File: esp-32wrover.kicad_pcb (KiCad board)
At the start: 2 copper layers, 68.6 x 53.3 mm, 8 parts, among them P1 Power, P2 Analog, P3 Digital, P4 Digital, P5 CONN_1, P6 CONN_1, P7 CONN_1, P8 CONN_1

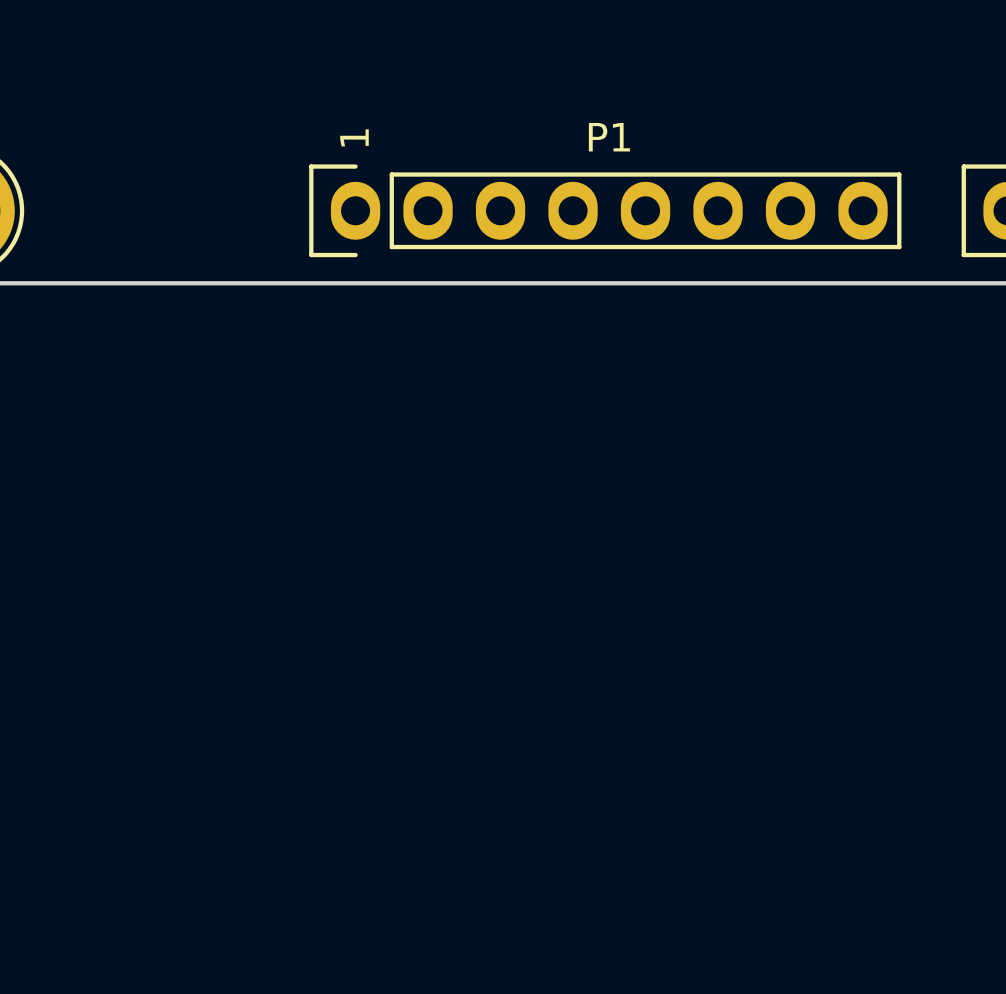
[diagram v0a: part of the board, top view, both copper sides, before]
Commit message: edit netlist, create pcb
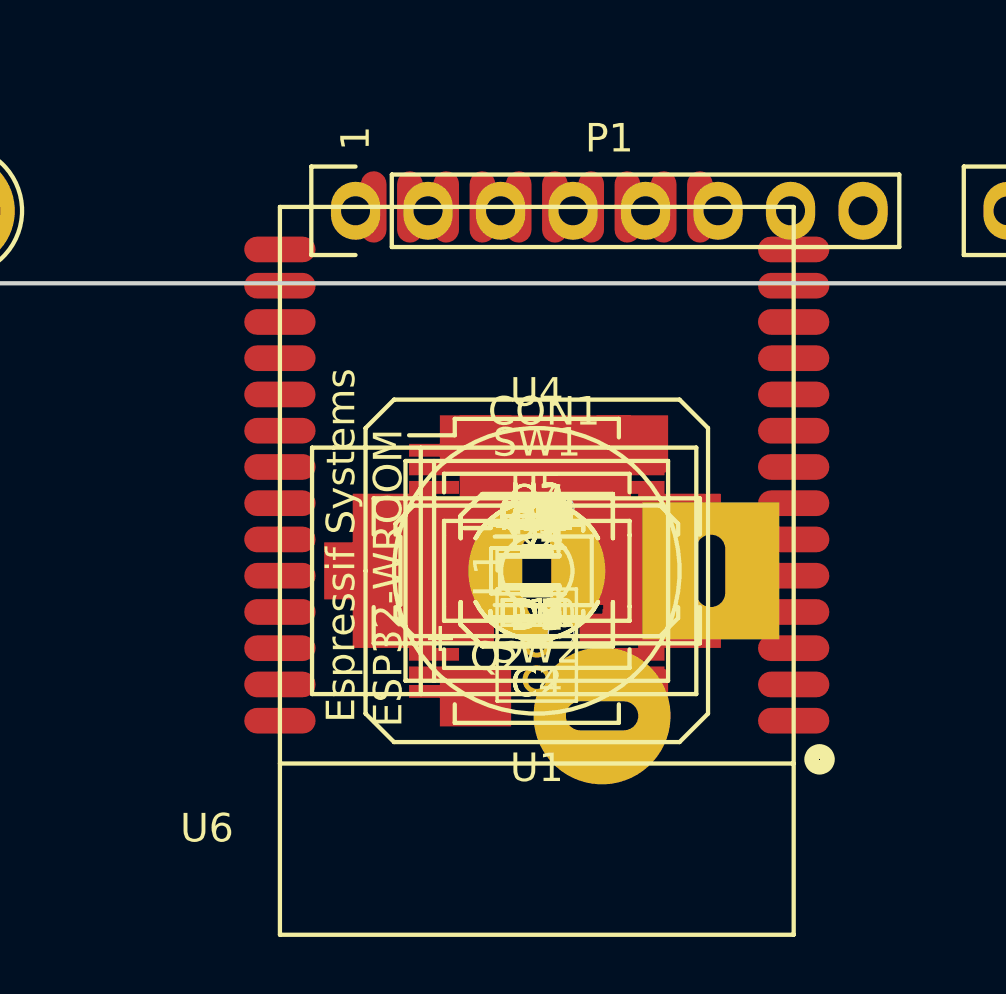
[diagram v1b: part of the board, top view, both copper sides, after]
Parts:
- added C1, C3: 1nF/50V, Capacitors_SMD:C_0603, F.Cu at (145.3, 136.4)
- added C10: 1uF, Capacitors_SMD:C_0805, F.Cu at (145.3, 136.4)
- added C11, C13, C14, C16, C17: C, Capacitors_SMD:C_0603, F.Cu at (145.3, 136.4)
- added C12, C15: 10uF/25V, Capacitors_SMD:C_0603, F.Cu at (145.3, 136.4)
- added C18: 1uF/25V, Capacitors_SMD:C_0603, F.Cu at (145.3, 136.4)
- added C19, C20: 0.1uF, Capacitors_SMD:C_0603, F.Cu at (145.3, 136.4)
- added C2, C4: 10uF/25V, Capacitors_SMD:c_elec_5x5.3, F.Cu at (145.3, 136.4)
- added C21: 100nF, Capacitors_SMD:C_0805, F.Cu at (145.3, 136.4)
- added C5: 10uF, Capacitors_SMD:C_0603, F.Cu at (145.3, 136.4)
- added C6: 1uF, Capacitors_SMD:C_0603, F.Cu at (145.3, 136.4)
- added C7, C8: 33pF, Capacitors_SMD:C_0603, F.Cu at (145.3, 136.4)
- added C9: 100nF, Capacitors_SMD:C_0603, F.Cu at (145.3, 136.4)
- added CON1: BARREL_JACK, Connect:JACK_ALIM, F.Cu at (145.3, 136.4)
- added D1, D3: D_Schottky_Small, Diodes_SMD:D_0805, F.Cu at (145.3, 136.4)
- added D10, D11, D6, D7, D8, D9: ZENER_3.3V, Diodes_SMD:D_0603, F.Cu at (145.3, 136.4)
- added D2: L_PWR, LEDs:LED_0603, F.Cu at (145.3, 136.4)
- added D4: L-RX, LEDs:LED_0603, F.Cu at (145.3, 136.4)
- added D5: L-TX, LEDs:LED_0603, F.Cu at (145.3, 136.4)
- added L1: 22uH, Inductors:SELF-WE-PD-XXL, F.Cu at (145.3, 136.4)
- added P9: CONN_01X04, Pin_Headers:Pin_Header_Straight_1x04_Pitch1.27mm, F.Cu at (145.3, 136.4)
- added Q1: 12Mhz, Crystals:Q_49U3HMS, F.Cu at (145.3, 136.4)
- added Q2: 32.768Khz, Crystals:Crystal_SMD_Micro-Crystal_MS1V-T1K, F.Cu at (145.3, 136.4)
- added Q3, Q4: Q_NPN_BEC, TO_SOT_Packages_SMD:SOT-23, F.Cu at (145.3, 136.4)
- added R1, R13, R14, R16, R2, R21, R22: 470R, Resistors_SMD:R_0603, F.Cu at (145.3, 136.4)
- added R10: 10k, Resistors_SMD:R_0603, F.Cu at (145.3, 136.4)
- added R11: 3K, Resistors_SMD:R_0603, F.Cu at (145.3, 136.4)
- added R12, R19, R20: 1K, Resistors_SMD:R_0603, F.Cu at (145.3, 136.4)
- added R15: 4K7, Resistors_SMD:R_0603, F.Cu at (145.3, 136.4)
- added R17, R18, R6, R7, R8: 10K, Resistors_SMD:R_0603, F.Cu at (145.3, 136.4)
- added R23, R25, R27, R29, R31, R33: 220k/1%, Resistors_SMD:R_0603, F.Cu at (145.3, 136.4)
- added R24, R26, R28, R30, R32, R34: 100k, Resistors_SMD:R_0603, F.Cu at (145.3, 136.4)
- added R3, R4: 27R, Resistors_SMD:R_0603, F.Cu at (145.3, 136.4)
- added R5: 1.5K, Resistors_SMD:R_0603, F.Cu at (145.3, 136.4)
- added R9: 52.5K, Resistors_SMD:R_0603, F.Cu at (145.3, 136.4)
- added SW1: SW_PUSH, Buttons_Switches_SMD:SW_SPST_B3SL-1022P, F.Cu at (145.3, 136.4)
- added SW2: SW_PUSH, Buttons_Switches_SMD:SW_SPST_REED_CT05-XXXX-G1, F.Cu at (145.3, 136.4)
- added U1: usb_mini_b, Connect:USB_Mini-B, F.Cu at (145.3, 136.4)
- added U2: MCP16311-MNY, Housings_SSOP:MSOP-8-1EP_3x3mm_Pitch0.65mm, F.Cu at (145.3, 136.4)
- added U3: BD00GA5WEFJ, Housings_SSOP:MSOP-8-1EP_3x3mm_Pitch0.65mm, F.Cu at (145.3, 136.4)
- added U4: PL2303HXA, Housings_SSOP:SSOP-28_5.3x10.2mm_Pitch0.65mm, F.Cu at (145.3, 136.4)
- added U5: MCP6001R, TO_SOT_Packages_SMD:SOT-23-5, F.Cu at (145.3, 136.4)
- added U6: ESP32-WROVER, ESP32-footprints-Lib:ESP32-WROOM, F.Cu at (145.3, 136.4)
- added U7: IRLM6402, TO_SOT_Packages_SMD:SOT-23, F.Cu at (145.3, 136.4)
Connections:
- P1 pad 3: /Reset -> EN
- P1 pad 8: /Vin -> Vin
- P2 pad 1: /A0 -> A0
- P2 pad 2: /A1 -> A1
- P2 pad 3: /A2 -> A2
- P2 pad 4: /A3 -> A4
- P2 pad 5: /A4(SDA) -> A5
- P2 pad 6: /A5(SCL) -> A6
- P3 pad 1: /A5(SCL) -> CMD
- P3 pad 10: /8 -> IO27
- P3 pad 2: /A4(SDA) -> CLK
- P3 pad 3: /AREF -> SDO
- P3 pad 5: /13(SCK) -> SD1
- P3 pad 6: /12(MISO) -> SD2
- P3 pad 7: /11(**/MOSI) -> SD3
- P3 pad 8: /10(**/SS) -> IO17
- P3 pad 9: /9(**) -> IO16
- P4 pad 1: /7 -> RXD
- P4 pad 2: /6(**) -> TXD
- P4 pad 3: /5(**) -> GPIO0
- P4 pad 4: /4 -> GPIO2
- P4 pad 5: /3(**) -> IO12
- P4 pad 6: /2 -> IO13
- P4 pad 7: /1(Tx) -> IO14
- P4 pad 8: /0(Rx) -> IO15
